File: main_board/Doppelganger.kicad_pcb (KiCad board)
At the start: 2 copper layers, 76.1 x 51.9 mm, 70 parts, among them J1 RJ45, J2 dnf, J3 dnf, P1 BORNIER_10, P2 BORNIER_10, P3 CONN_01X06, P4 CONN_01X06, P5 TTL Serial, P6 Status Leds, SW1 SW_PUSH, SW2 SW_PUSH, U1 74HC32, U2 SIP32510, U4 74LVC07, U5 74LVC07, U6 74LVC07, U8 18F45K50, U9 MAX4737

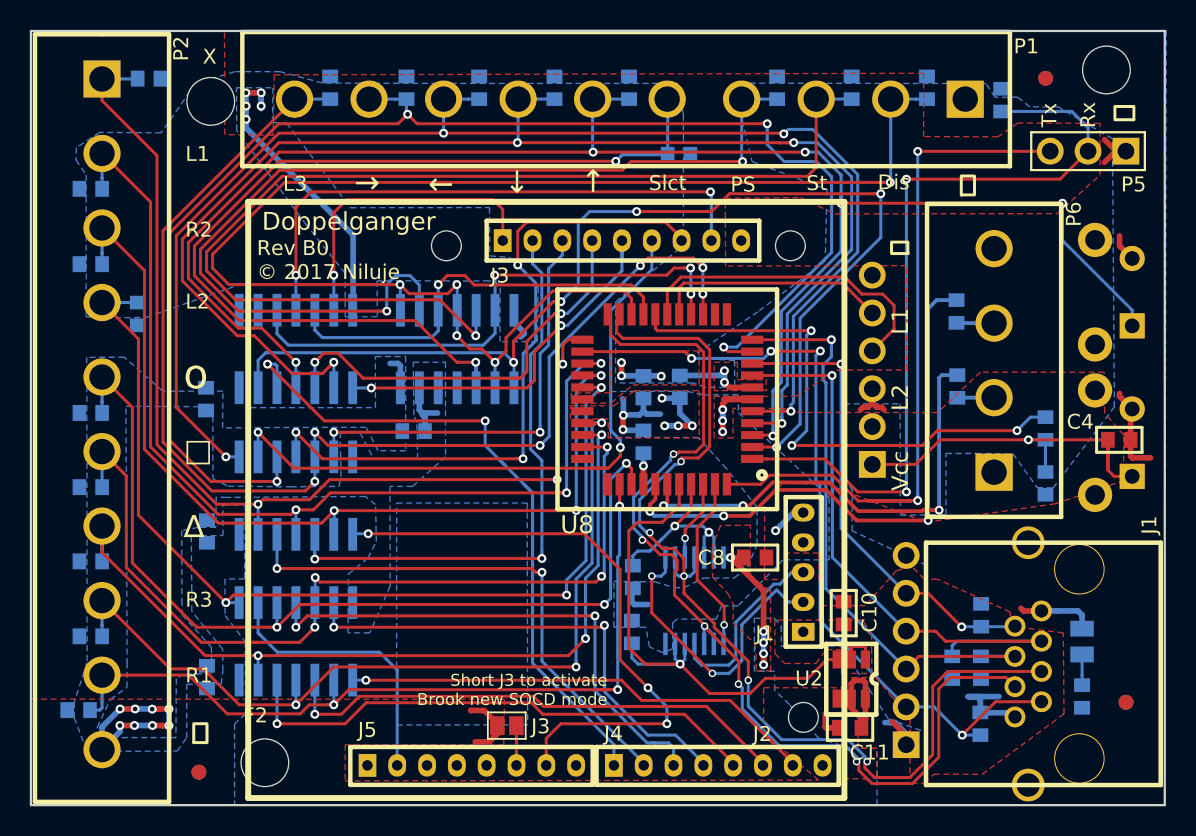
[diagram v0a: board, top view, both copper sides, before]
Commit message: RevB0
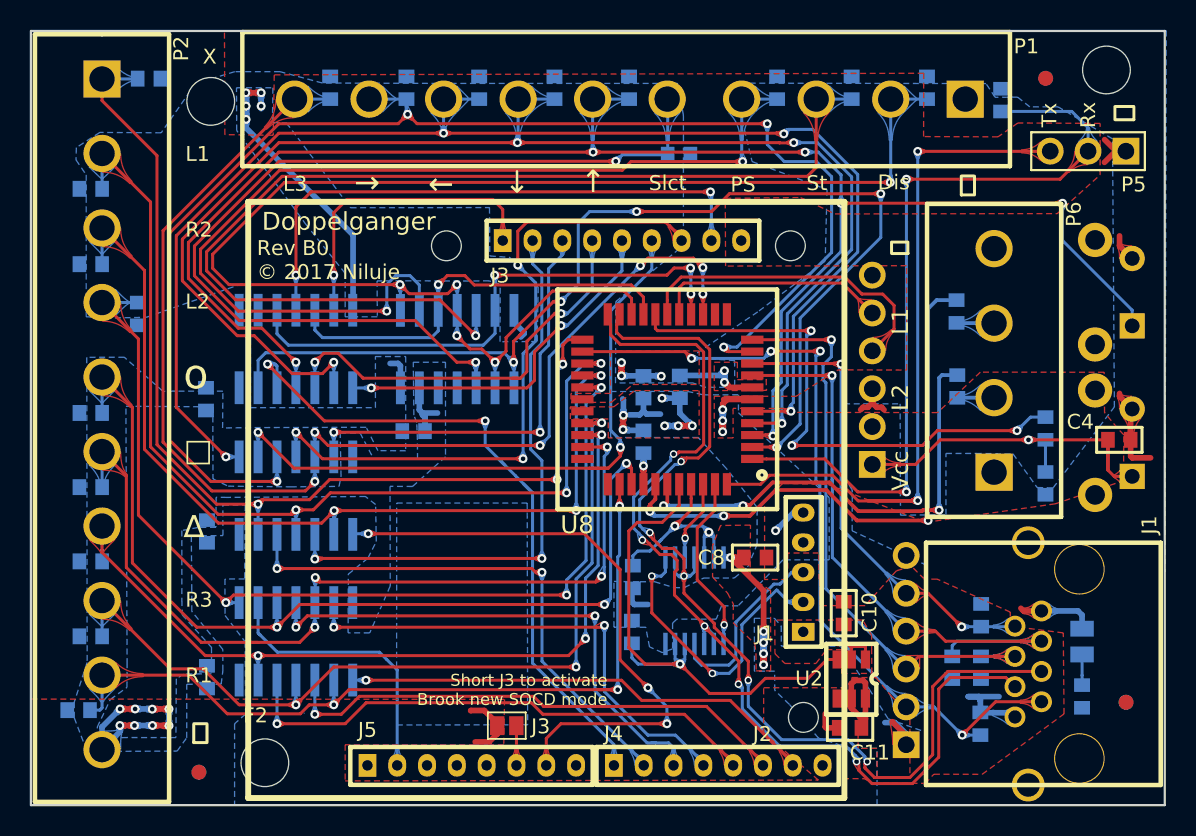
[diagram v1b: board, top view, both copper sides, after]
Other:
- net class Leds: clearance 0.254 -> 0.2032
- rule trace_min: 0.1524 -> 0.2032
